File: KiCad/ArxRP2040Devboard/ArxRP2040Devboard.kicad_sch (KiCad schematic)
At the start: 32 parts, among them J1 USB_C_Receptacle_USB2.0_14P, J2 Conn_01x03, J3 Conn_01x20, J4 Conn_01x20, SW1 SW_Push, U1 NCP1117-1.5_SOT223, U2 RP2040, U3 W25Q128JVS, Y1 Crystal_GND24

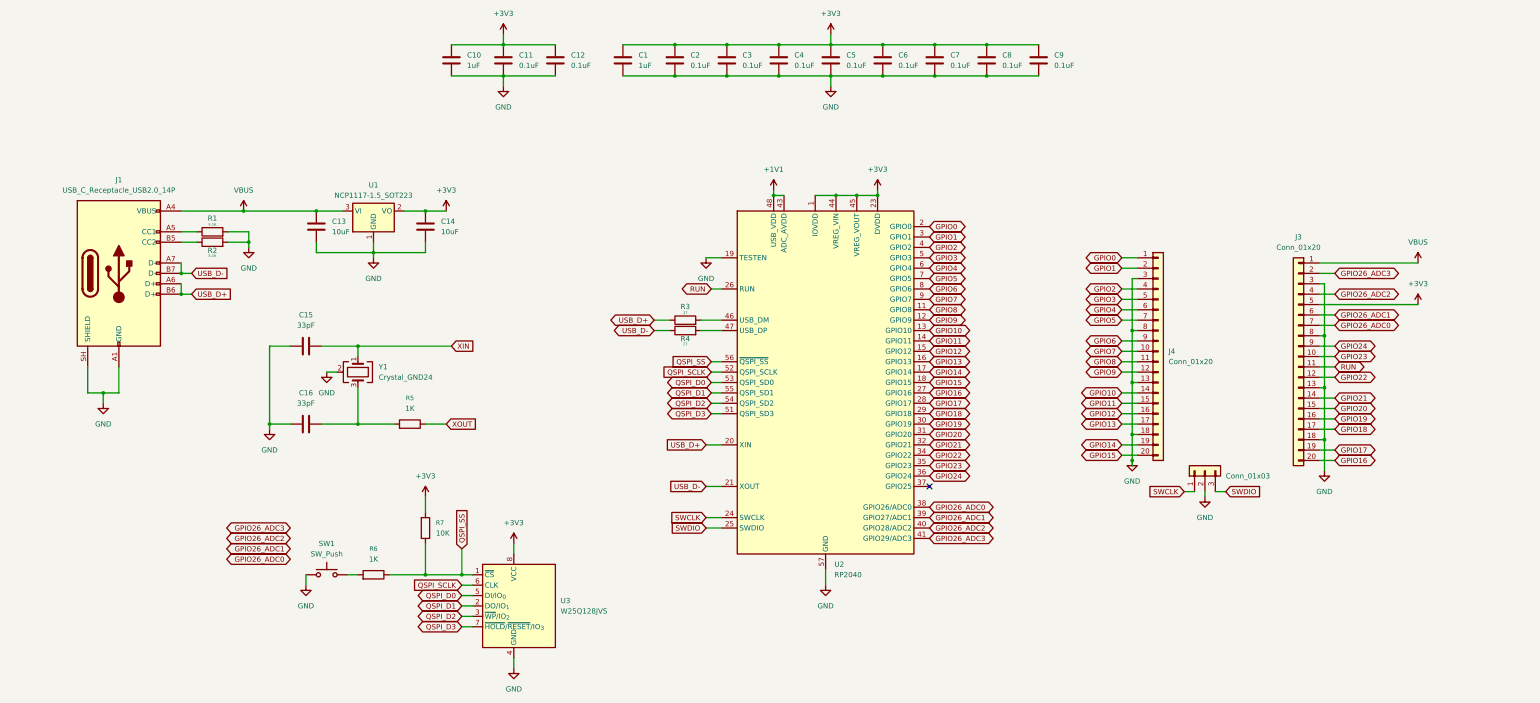
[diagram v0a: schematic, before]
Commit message: schematics
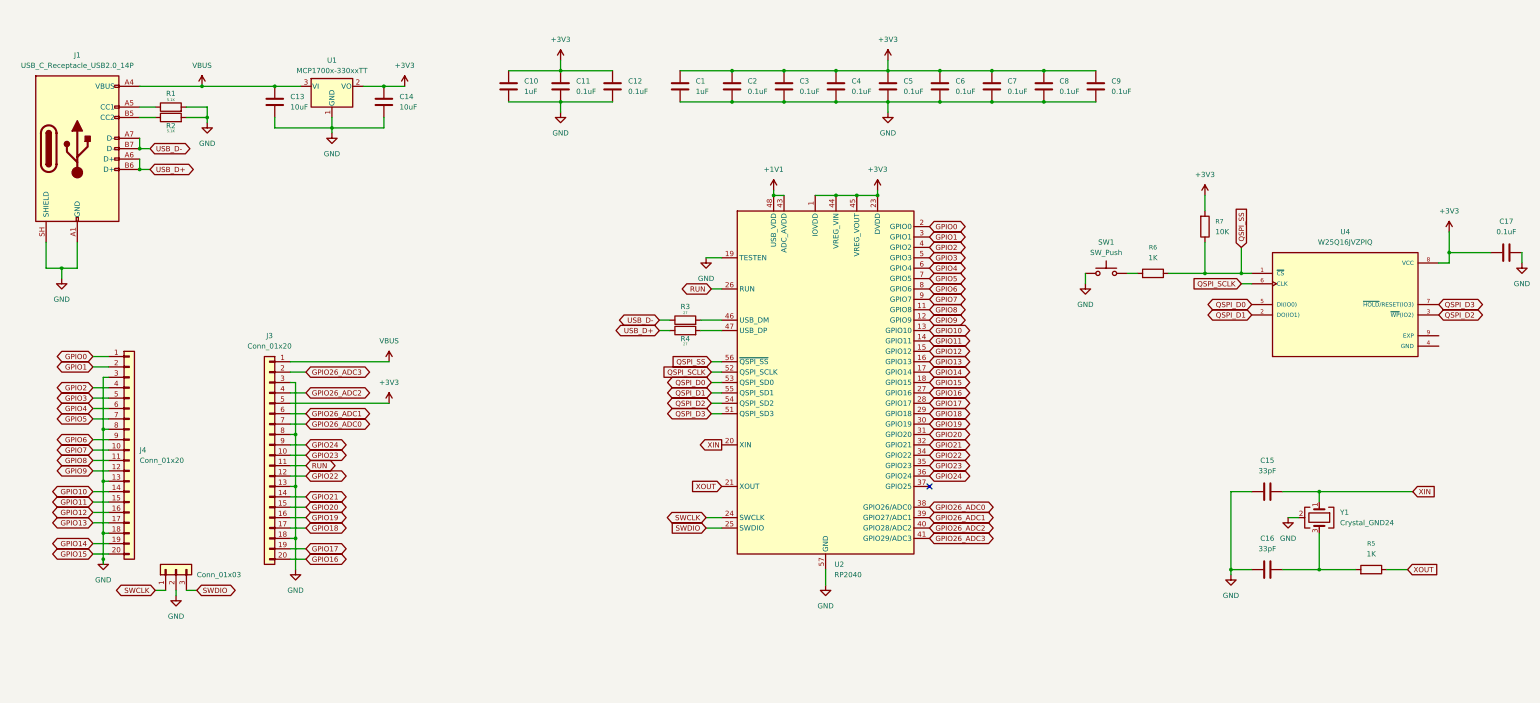
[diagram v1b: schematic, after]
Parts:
- removed U1: NCP1117-1.5_SOT223, Package_TO_SOT_SMD:SOT-223-3_TabPin2, symbol Regulator_Linear:NCP1117-1.5_SOT223
- removed U3: W25Q128JVS, Package_SO:SOIC-8_5.3x5.3mm_P1.27mm, symbol Memory_Flash:W25Q128JVS
- added C17: 0.1uF, Capacitor_SMD:C_0402_1005Metric, symbol Device:C
- added U1: MCP1700x-330xxTT, Package_TO_SOT_SMD:SOT-23, symbol Regulator_Linear:MCP1700x-330xxTT
- added U4: W25Q16JVZPIQ, Package_SON:Winbond_USON-8-1EP_3x2mm_P0.5mm_EP0.2x1.6mm, symbol W25Q16JVZPIQ:W25Q16JVZPIQ
- C13, C14: footprint Capacitor_SMD:C_0201_0603Metric -> Capacitor_SMD:C_0603_1608Metric
- J1: footprint (none) -> Connector_USB:USB_C_Receptacle_HRO_TYPE-C-31-M-12
- J2: footprint (none) -> Connector_PinHeader_2.54mm:PinHeader_1x03_P2.54mm_Vertical
- J3, J4: footprint (none) -> Connector_PinHeader_2.54mm:PinHeader_1x20_P2.54mm_Vertical
- R1, R2, R3, R4, R5, R6, R7: footprint (none) -> Resistor_SMD:R_0402_1005Metric
- SW1: footprint (none) -> Button_Switch_SMD:SW_Push_SPST_NO_Alps_SKRK
- Y1: footprint (none) -> Crystal:Crystal_SMD_3225-4Pin_3.2x2.5mm_HandSoldering
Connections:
- net +3V3: now also C17.1, U1.2 (VO), U4.8 (VCC)
- net GND: now also C17.2, U1.1 (GND)
- net QSPI_D0: now also U4.5 (DI(IO0))
- net QSPI_D1: now also U4.2 (DO(IO1))
- net QSPI_D2: now also U4.3 (~{WP}(IO2))
- net QSPI_D3: now also U4.7 (~{HOLD}/RESET(IO3))
- net QSPI_SCLK: now also U4.6 (CLK)
- net QSPI_SS: now also U4.1 (~{CS})
- net USB_D+: now also R4.1; no longer R3.1, U2.20 (XIN)
- net USB_D-: now also R3.1; no longer R4.1, U2.21 (XOUT)
- net VBUS: now also U1.3 (VI)
- net XIN: now also U2.20 (XIN)
- net XOUT: now also U2.21 (XOUT)
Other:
- moved on the sheet: C1, C10, C11, C12, C13, C14, C15, C16, C2, C3, C4, C5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
